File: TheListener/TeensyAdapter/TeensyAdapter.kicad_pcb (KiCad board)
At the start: 2 copper layers, 21 parts, among them J1 Conn_02x05_Odd_Even, J2 Conn_02x05_Odd_Even, J3 Conn_01x04_Male, J4 Conn_01x04_Male, U1 Teensy3.5

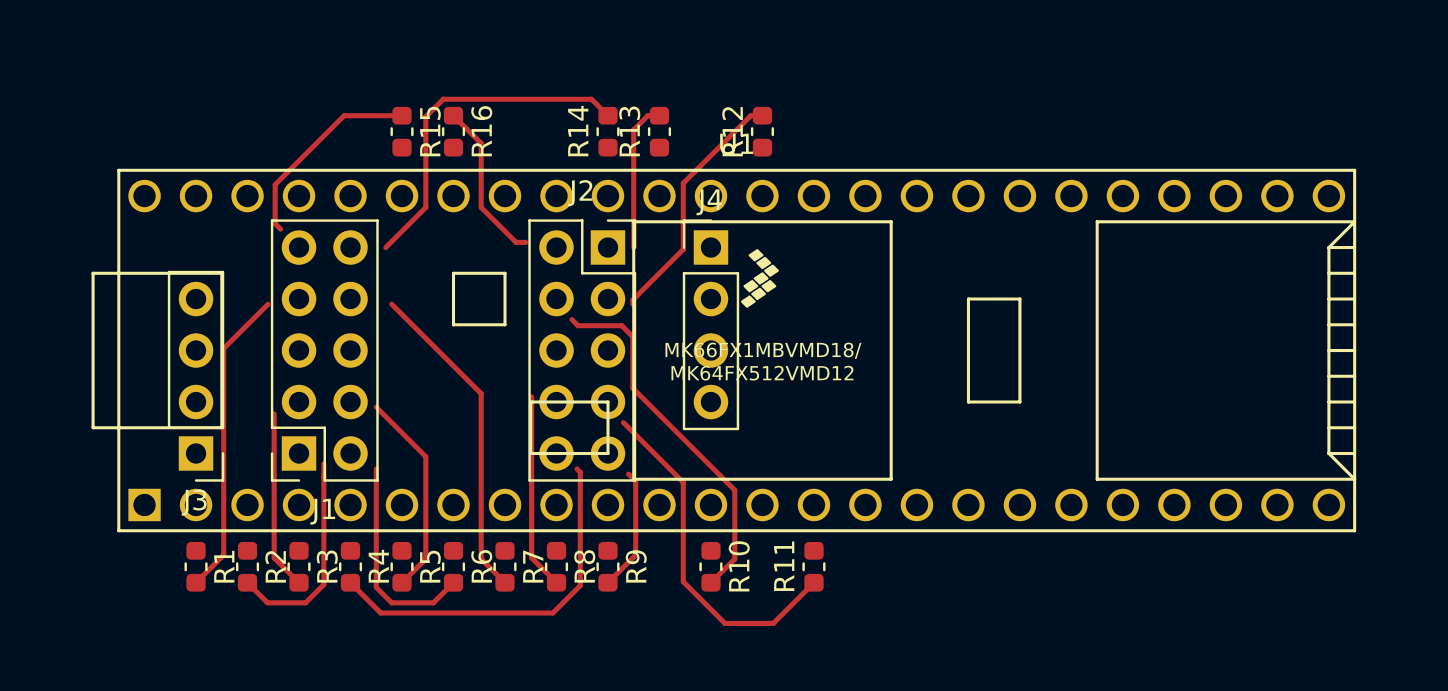
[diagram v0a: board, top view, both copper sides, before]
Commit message: updates
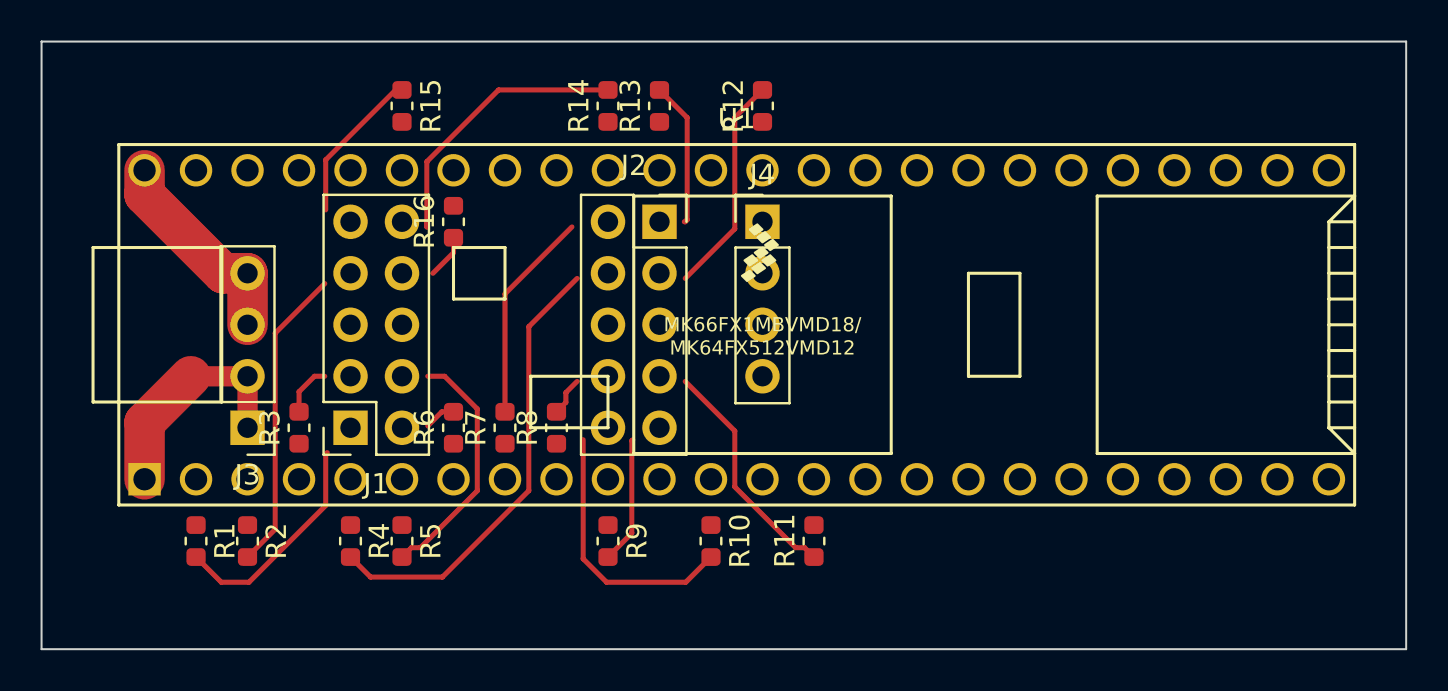
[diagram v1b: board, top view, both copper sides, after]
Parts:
- moved R3 6.86 mm to (149.9, 138.4), turned to 90 degrees
- moved R6 6.86 mm to (157.5, 138.4), turned to 90 degrees
- moved R7 6.86 mm to (160.0, 138.4), turned to 90 degrees
- moved R8 6.86 mm to (162.6, 138.4), turned to 90 degrees
- moved R16 4.45 mm to (157.5, 128.3), turned to 90 degrees
- moved J1 2.84 mm to (152.4, 138.4)
- moved J2 2.84 mm to (167.6, 128.3)
- moved J3 2.84 mm to (147.3, 138.4)
- moved J4 2.84 mm to (172.7, 128.3)
- moved R1 1.27 mm to (144.8, 144.0)
- moved R10 1.27 mm to (170.2, 144.0)
- moved R11 1.27 mm to (175.3, 144.0)
- moved R2 1.27 mm to (147.3, 144.0)
- moved R4 1.27 mm to (152.4, 144.0)
- moved R5 1.27 mm to (154.9, 144.0)
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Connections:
- U1 pad 1: (no net) -> GND
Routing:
- net GND: track 0.00 -> 11.4 mm
- net +5V: track 0.00 -> 10.4 mm
- net T_2: track 10.4 -> 1.56 mm
- net T_6: track 9.68 -> 1.92 mm
- net T_1: track 8.83 -> 2.58 mm
- net T_7: track 8.00 -> 2.17 mm
- net R_4: track 17.2 -> 11.6 mm
- net T_3: track 16.1 -> 10.5 mm
- net R_3: track 18.1 -> 13.2 mm
- net R_7: track 10.5 -> 15.1 mm
- net R_1: track 18.3 -> 22.4 mm
- net R_8: track 15.2 -> 11.1 mm
- net R_6: track 16.9 -> 13.9 mm
- net T_8: track 9.97 -> 7.66 mm
- net R_2: track 10.2 -> 12.2 mm
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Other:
- board outline added: 67.3 x 30 mm
